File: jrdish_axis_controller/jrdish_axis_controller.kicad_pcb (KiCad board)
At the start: 2 copper layers, 114 parts, among them CN1 KF2EDGR-2.54-9P, CN2 KF2EDGR-2.54-6P, CN3 KF2EDGR-2.54-4P, CN4 KF2EDGR-2.54-4P, CN5 KF2EDGR-2.54-2P, CN6 KF2EDGR-2.54-2P, CN7 SM04B-SRSS-TB (LF)(SN), CN8 SM04B-SRSS-TB (LF)(SN), J1 Conn_ARM_SWD_TagConnect_TC2030, M1 MountingHole_2.7mm_M2.5_ISO14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, Q1 AO3407A, Q2 AO3400A, SW1 DSHP04TSGER, SW2 SS-12F49-G050, U1 STM32G474CET6, U2 ISOW1432BDFMR, U3 MP2322GQH-Z, U4 LTC4311ISC6#TRPBF, U5 LM75BIMX-5/NOPB, U6 M24C64-RMN6TP, X1 NX2016SA-16MHZ-EXS00A-CS07826

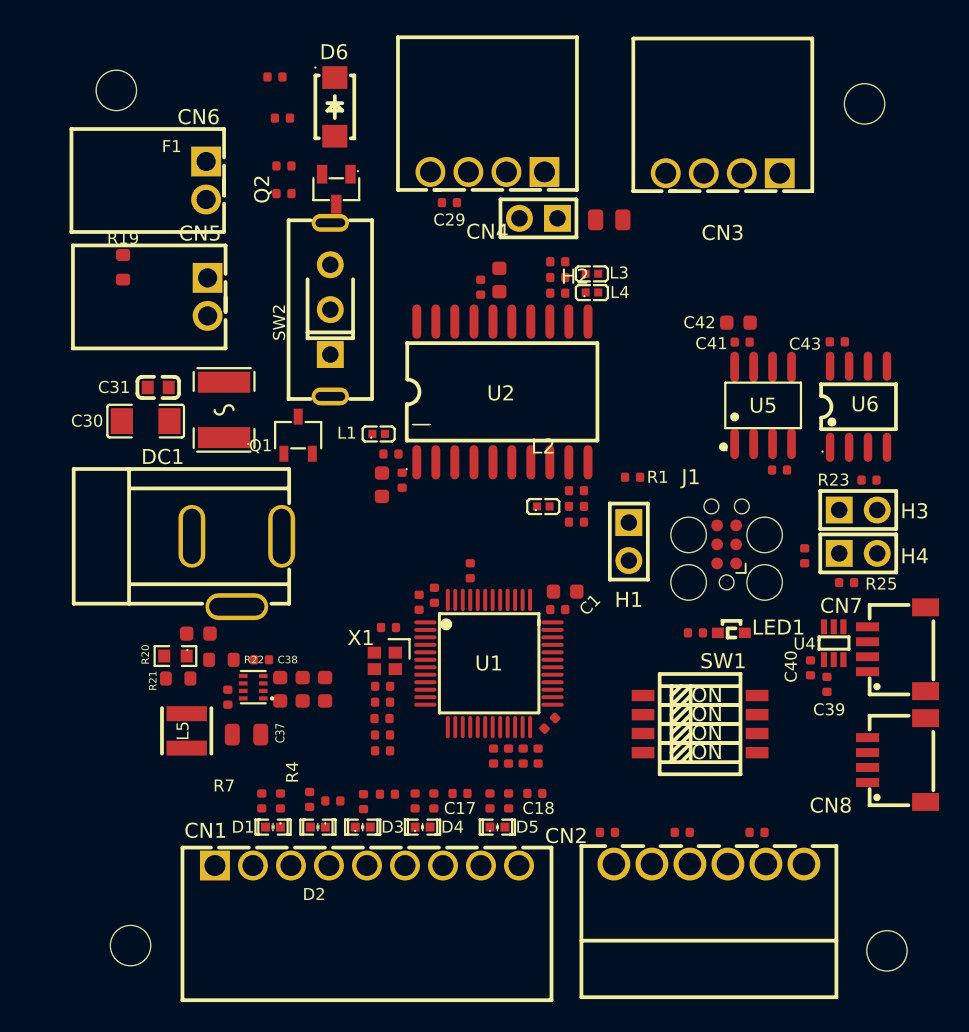
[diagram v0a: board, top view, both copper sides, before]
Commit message: PCB layout in progress
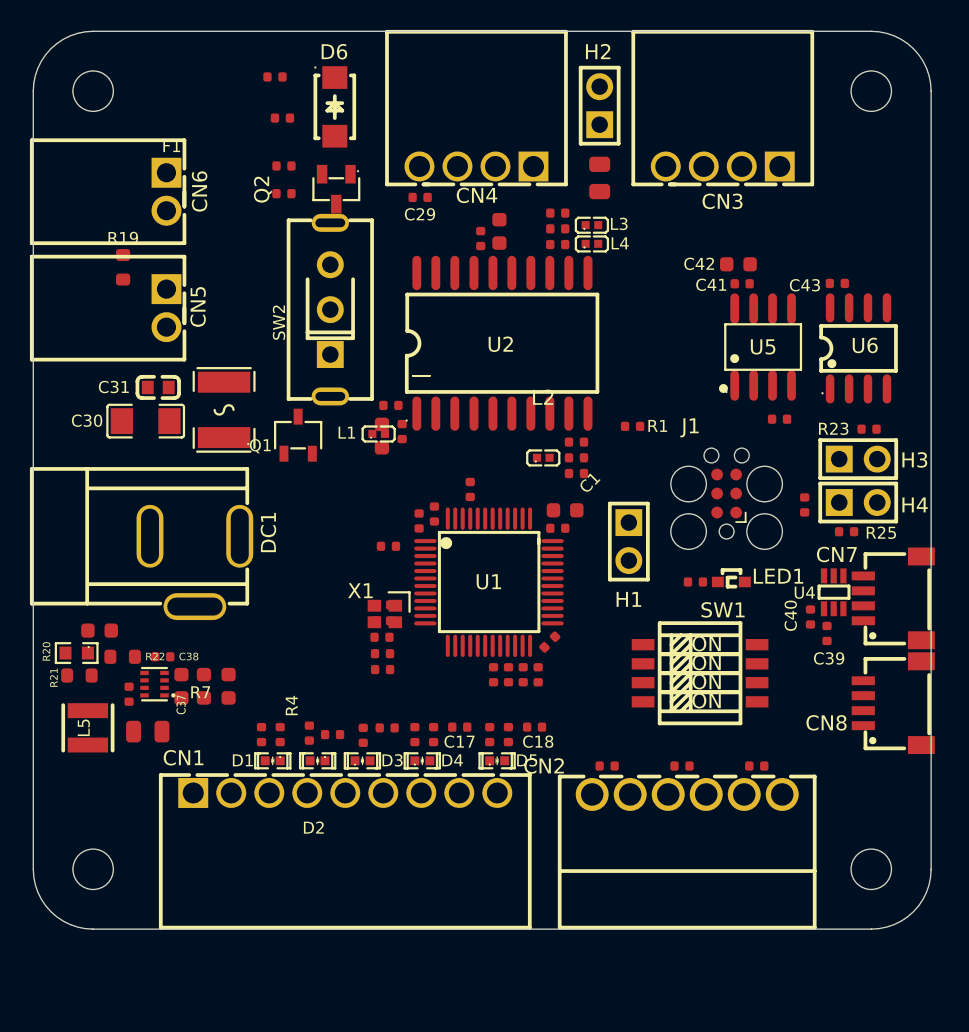
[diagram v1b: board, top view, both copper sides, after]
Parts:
- moved H2 8.57 mm to (163.5, 75.7), turned to 90 degrees
- moved R21 6.60 mm to (128.7, 113.7)
- moved C32 6.60 mm to (132.1, 115.0)
- moved C34 6.60 mm to (137.1, 114.5)
- moved C35 6.60 mm to (135.6, 114.5)
- moved C36 6.60 mm to (130.1, 110.7)
- moved C37 6.60 mm to (133.3, 117.5)
- moved C38 6.60 mm to (134.3, 112.5)
- moved L5 6.60 mm to (129.3, 117.2)
- moved R20 6.60 mm to (128.6, 112.2)
- moved R22 6.60 mm to (131.6, 112.5)
- moved U3 6.60 mm to (133.8, 114.3)
- moved C33 6.45 mm to (138.7, 114.5)
- moved M1 5.68 mm to (129.7, 126.7)
- moved M1 5.55 mm to (181.7, 126.7)
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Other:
- board outline added: 60 x 60 mm
